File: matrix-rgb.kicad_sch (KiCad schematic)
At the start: 33 parts

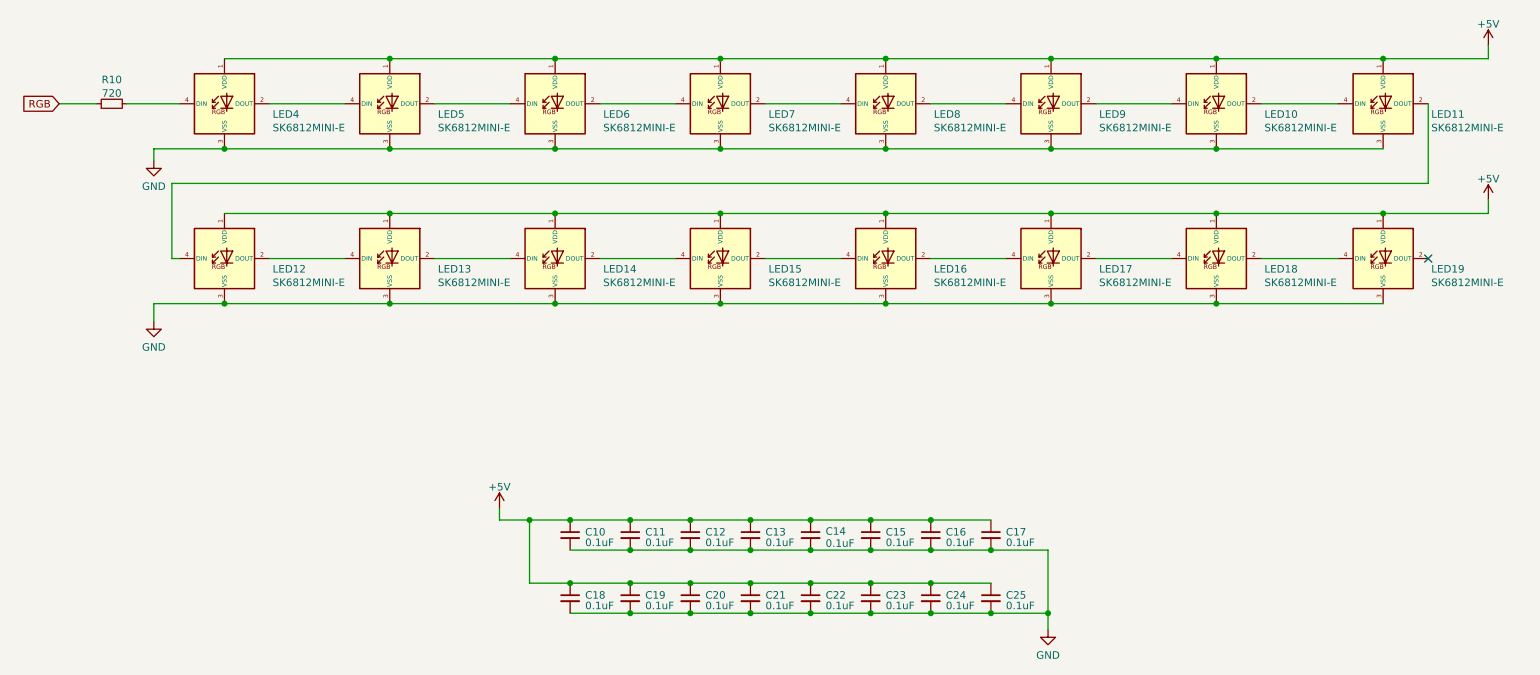
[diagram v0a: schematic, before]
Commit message: added MOAR LEDZZZZZZZZZ
5 more to be exact.
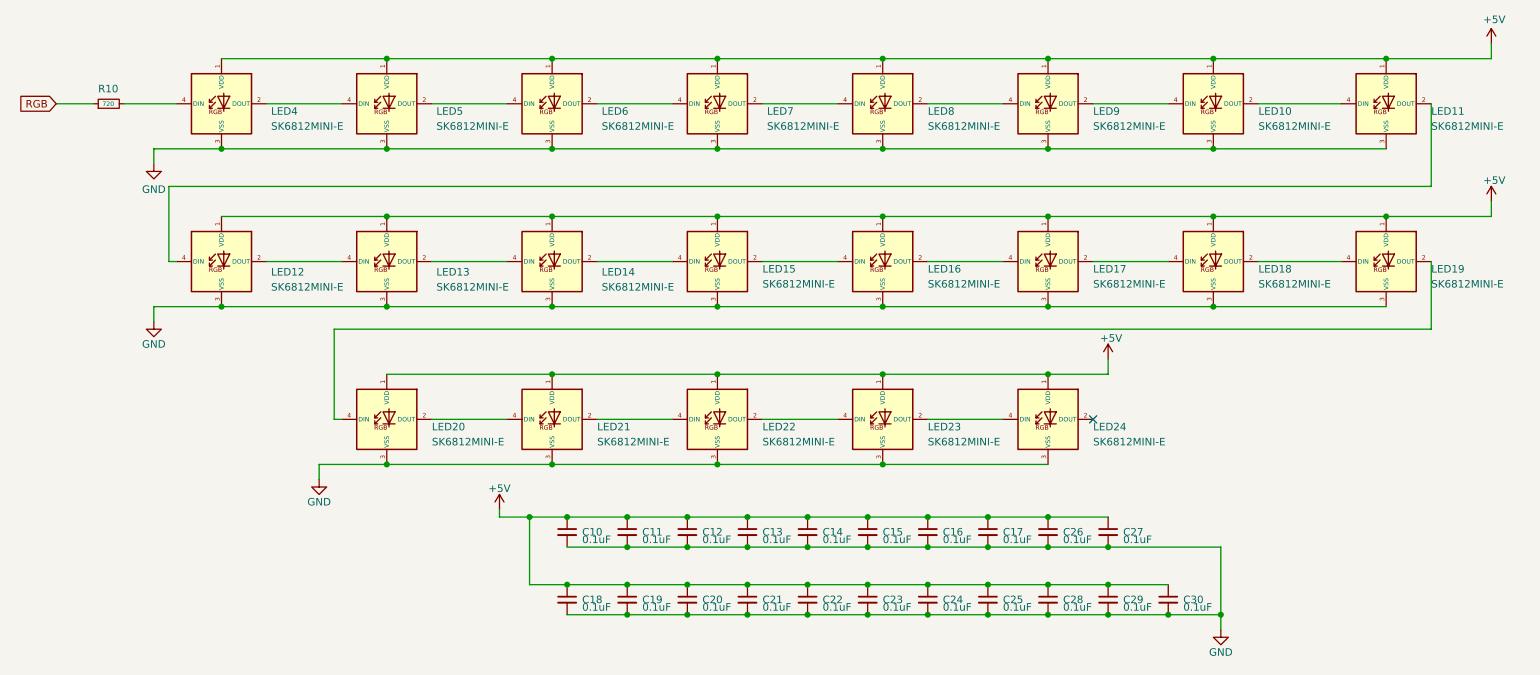
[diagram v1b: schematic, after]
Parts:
- added C26, C27, C28, C29, C30: 0.1uF, arisutea:C_0805_2012Metric_Pad1.18x1.45mm_HandSolder, symbol arisutea-pcb:Device_C_Small
- added LED20, LED21, LED22, LED23, LED24: SK6812MINI-E, arisutea:LED_SK6812MINI-E, symbol arisutea-pcb:LED_SK6812MINI-E
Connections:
- net +5V: now also C26.1, C27.1, C28.1, C29.1, C30.1, LED20.1 (VDD), LED21.1 (VDD), LED22.1 (VDD), LED23.1 (VDD), LED24.1 (VDD)
- net GND: now also C26.2, C27.2, C28.2, C29.2, C30.2, LED20.3 (VSS), LED21.3 (VSS), LED22.3 (VSS), LED23.3 (VSS), LED24.3 (VSS)
- net at LED19.2 (DOUT): now also LED20.4 (DIN)
- new net: LED22.2 (DOUT), LED23.4 (DIN)
- new net: LED21.2 (DOUT), LED22.4 (DIN)
- new net: LED23.2 (DOUT), LED24.4 (DIN)
- new net: LED20.2 (DOUT), LED21.4 (DIN)
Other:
- moved on the sheet: C10, C11, C12, C13, C14, C15, C16, C17, C18, C19, C20, C21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
